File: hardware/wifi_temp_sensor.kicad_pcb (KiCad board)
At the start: 2 copper layers, 50.8 x 45.7 mm, 12 parts, among them J1 USB_B_Mini, J2 ESP8266, J3 TempSensor, J4 Prog, J5 Aux_I2C, SW1 BootMode, U2 AZ1117-3.3

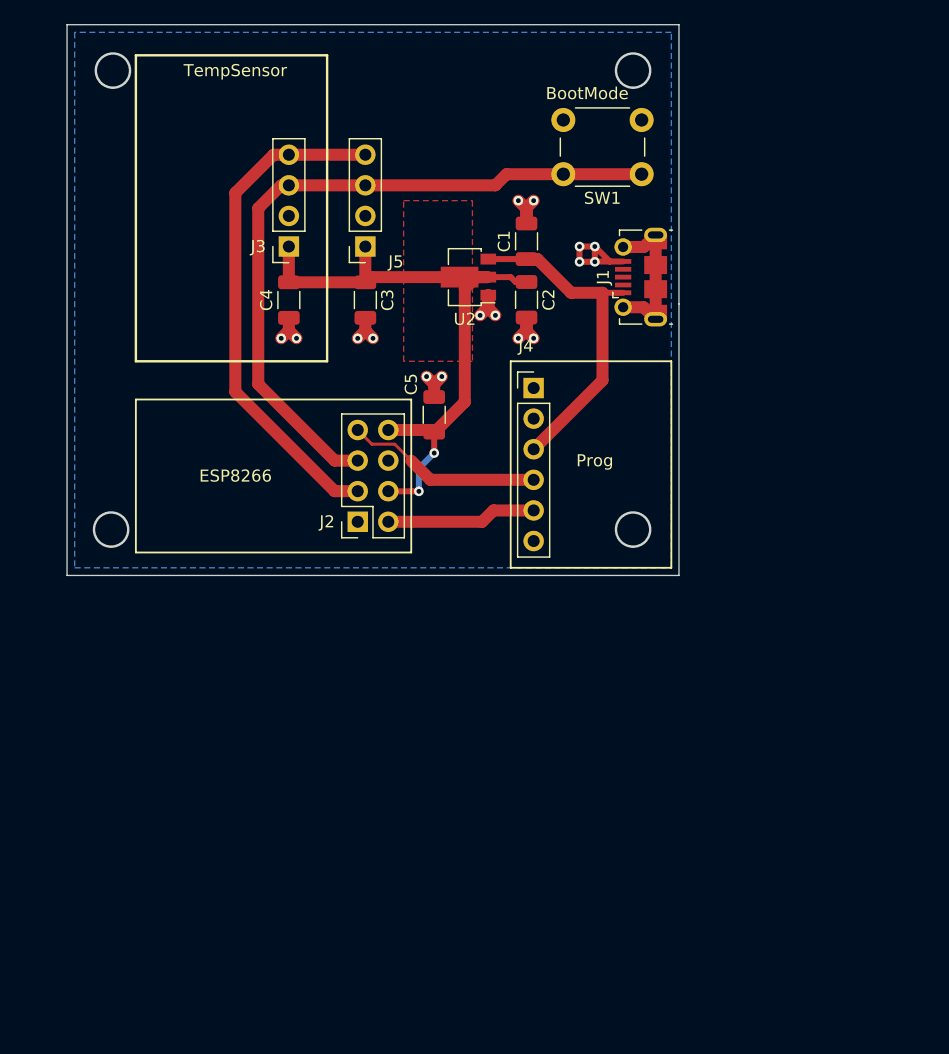
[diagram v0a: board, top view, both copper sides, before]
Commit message: manual merge from esp32_msf_rcnotes
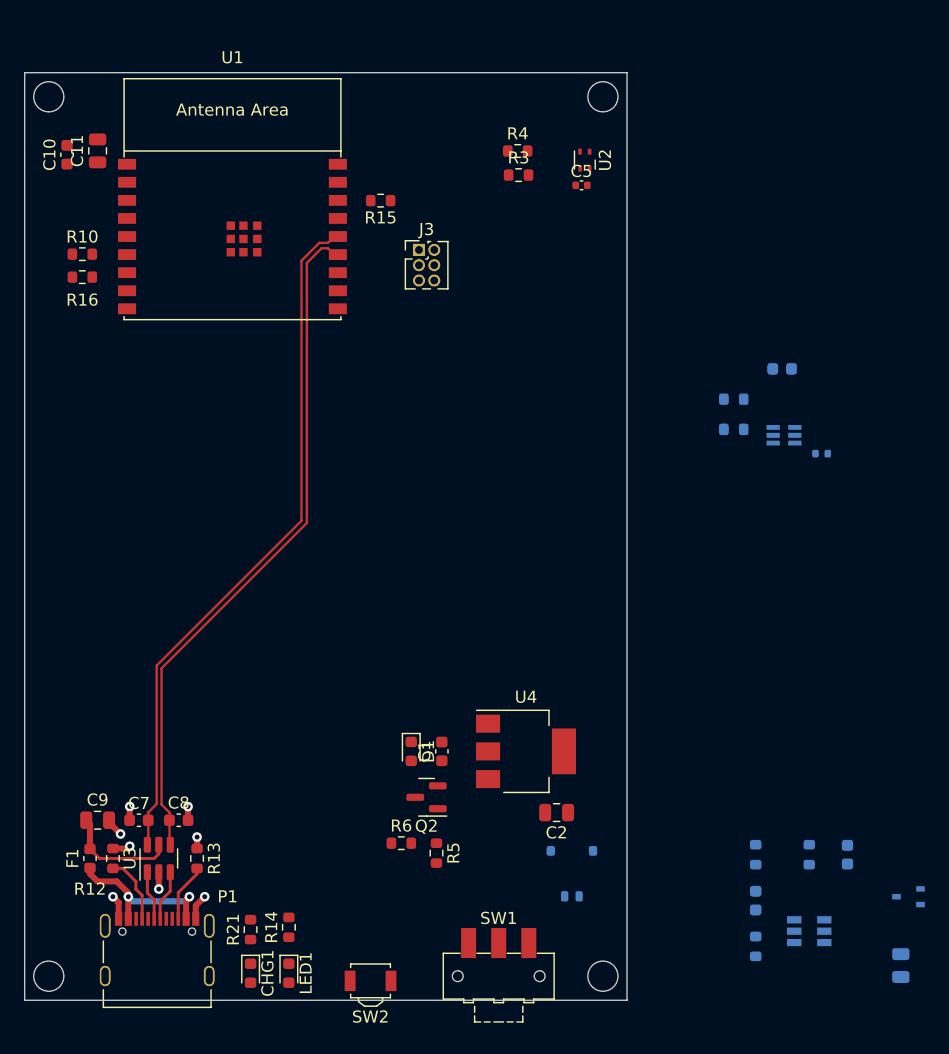
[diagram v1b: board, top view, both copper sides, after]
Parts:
- removed J1: USB_B_Mini, Connector_USB:USB_Micro-B_Molex-105017-0001
- removed J4: Prog, Connector_PinHeader_2.54mm:PinHeader_1x06_P2.54mm_Vertical
- removed J5: Aux_I2C, Connector_PinSocket_2.54mm:PinSocket_1x04_P2.54mm_Vertical
- added C10: 100nF, Capacitor_SMD:C_0603_1608Metric, F.Cu at (183.5, 35.6)
- added C11: 10uF, Capacitor_SMD:C_0805_2012Metric, F.Cu at (186.1, 35.2)
- added C12: 100nF, Capacitor_SMD:C_0603_1608Metric, B.Cu at (248.3, 93.7)
- added C6: 10uF, Capacitor_SMD:C_0805_2012Metric, B.Cu at (252.7, 102.9)
- added C7: 22pF, Capacitor_SMD:C_0603_1608Metric, F.Cu at (189.5, 90.8)
- added C8: 22pF, Capacitor_SMD:C_0603_1608Metric, F.Cu at (192.8, 90.8)
- added C9: 10uF, Capacitor_SMD:C_0805_2012Metric, F.Cu at (186.1, 90.8)
- added CHG1: LED_Small, LED_SMD:LED_0603_1608Metric, F.Cu at (198.8, 103.5)
- added D1: D_Schottky, Diode_SMD:D_0603_1608Metric, F.Cu at (212.1, 85.1)
- added F1: Polyfuse_Small, Fuse:Fuse_0603_1608Metric, F.Cu at (185.4, 94.0)
- added IC2: BQ21040DBVR, TI BQ21040:SOT95P280X145-6N, B.Cu at (245.1, 100.0)
- added LED1: LED_Small, LED_SMD:LED_0603_1608Metric, F.Cu at (201.9, 103.5)
- added P1: USB_C_Plug_USB2.0, Connector_USB:USB_C_Receptacle_Palconn_UTC16-G, F.Cu at (191.0, 101.5)
- added Q1: SSM6L09FUTE85LF, SamacSys_parts:SOT65P210X120-6N, B.Cu at (243.0, 58.9)
- added Q2: AO3401A, Package_TO_SOT_SMD:SOT-23, F.Cu at (213.4, 88.9)
- added Q3: BSS214NW, Package_TO_SOT_SMD:SOT-323_SC-70, B.Cu at (253.4, 97.2)
- added R1: 100K, Resistor_SMD:R_0603_1608Metric, B.Cu at (238.9, 55.9)
- added R10: 10k, Resistor_SMD:R_0603_1608Metric, F.Cu at (184.8, 43.8)
- added R11: 100K, Resistor_SMD:R_0402_1005Metric, B.Cu at (246.2, 60.4)
- added R12: 5.1K, Resistor_SMD:R_0603_1608Metric, F.Cu at (187.3, 94.0)
- added R13: 5.1K, Resistor_SMD:R_0603_1608Metric, F.Cu at (194.3, 94.0)
- added R14: 33R, Resistor_SMD:R_0603_1608Metric, F.Cu at (201.9, 99.7)
- added R15: 10k, Resistor_SMD:R_0603_1608Metric, F.Cu at (209.6, 39.4)
- added R16: 10k, Resistor_SMD:R_0603_1608Metric, F.Cu at (184.8, 45.7)
- added R19: 33K, Resistor_SMD:R_0603_1608Metric, B.Cu at (240.7, 93.7)
- added R2: 100K, Resistor_SMD:R_0603_1608Metric, B.Cu at (238.9, 58.4)
- added R20: 10K, Resistor_SMD:R_0603_1608Metric, B.Cu at (245.1, 93.7)
- added R21: 33R, Resistor_SMD:R_0603_1608Metric, F.Cu at (198.8, 99.9)
- added R3: 10k, Resistor_SMD:R_0603_1608Metric, F.Cu at (221.0, 37.2)
- added R4: 10k, Resistor_SMD:R_0603_1608Metric, F.Cu at (220.9, 35.2)
- added R5: 10K, Resistor_SMD:R_0603_1608Metric, F.Cu at (214.2, 93.5)
- added R6: 1K, Resistor_SMD:R_0603_1608Metric, F.Cu at (211.3, 92.7)
- added R9: R_Small, Resistor_SMD:R_0603_1608Metric, B.Cu at (240.7, 101.3)
- added SW2: SW_Push, Button_Switch_SMD:SW_SPST_B3U-3000P, F.Cu at (208.7, 104.1)
- added U1: ESP32-C3-WROOM-02, PCM_Espressif:ESP32-C3-WROOM-02, F.Cu at (197.2, 42.2)
- added U3: WE-TVS-82400102, Package_TO_SOT_SMD:SOT-23-6, F.Cu at (191.1, 94.0)
- added U4: LD1117S33TR_SOT223, Package_TO_SOT_SMD:SOT-223-3_TabPin2, F.Cu at (221.6, 85.1)
- C1: value 10uF -> 1uF; footprint Capacitor_SMD:C_1206_3216Metric -> Capacitor_SMD:C_0603_1608Metric
- C2: value 22uF -> 10uF; footprint Capacitor_SMD:C_1206_3216Metric -> Capacitor_SMD:C_0805_2012Metric
- C3: value C_Small -> 1uF; footprint Capacitor_SMD:C_1206_3216Metric -> Capacitor_SMD:C_0603_1608Metric; moved to B.Cu
- C4: value C_Small -> 100nF; footprint Capacitor_SMD:C_1206_3216Metric -> Capacitor_SMD:C_0603_1608Metric; moved to B.Cu
- C5: value C_Small -> 100nF; footprint Capacitor_SMD:C_1206_3216Metric -> Capacitor_SMD:C_0402_1005Metric
- J2: value ESP8266 -> Batt_Conn; footprint Connector_PinSocket_2.54mm:PinSocket_2x04_P2.54mm_Vertical -> Connector_JST:JST_ACH_BM02B-ACHSS-GAN-ETF_1x02-1MP_P1.20mm_Vertical; moved to B.Cu
- J3: value TempSensor -> Conn_02x03_Odd_Even; footprint Connector_PinSocket_2.54mm:PinSocket_1x04_P2.54mm_Vertical -> Connector_PinHeader_1.27mm:PinHeader_2x03_P1.27mm_Vertical
- SW1: value BootMode -> SW_SPST; footprint Button_Switch_THT:SW_PUSH_6mm -> Button_Switch_SMD:SW_SPDT_CK-JS102011SAQN
- U2: value AZ1117-3.3 -> SHT4x; footprint Package_TO_SOT_SMD:SOT-89-3 -> Sensor_Humidity:Sensirion_DFN-4_1.5x1.5mm_P0.8mm_SHT4x_NoCentralPad
- moved SW1 67.6 mm to (219.3, 103.8), turned to 0 degrees
- moved C3 59.5 mm to (240.7, 97.5)
- moved C1 42.9 mm to (214.6, 85.1)
- moved C2 42.6 mm to (224.2, 90.2), turned to 180 degrees
- moved C4 41.3 mm to (242.9, 53.3), turned to 180 degrees
- moved J2 34.2 mm to (225.4, 95.2), turned to 0 degrees
- moved C5 22.6 mm to (226.2, 38.1), turned to 0 degrees
- moved U2 13.9 mm to (226.5, 36.0), turned to -90 degrees
- moved J3 10.8 mm to (212.7, 43.5), turned to 0 degrees
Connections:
- C1 pad 1: +5V -> Net-(D1-K)
- C3 pad 1: +3.3V -> V_USB
- C4 pad 1: GND -> V_BAT_MEAS
- C4 pad 2: +3.3V -> GND
- J2 pad 2: ESP_Tx -> Net-(J2-Pin_2)
- J3 pad 1: +3.3V -> EN
- J3 pad 2: GND -> +3.3V
- J3 pad 3: SCL -> TXD
- J3 pad 4: SDA -> IO9
- SW1 pad 1: SCL -> Net-(J2-Pin_2)
- SW1 pad 2: GND -> V_BAT
- U2 pad 1: GND -> SDA
- U2 pad 2: +3.3V -> SDC
- U2 pad 3: +5V -> +3.3V
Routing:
- net SCL: track 58.5 -> 0.00 mm
- net D+: track 0.00 -> 57.6 mm
- net D-: track 0.00 -> 56.9 mm
- net +3.3V: track 55.6 -> 0.00 mm, vias 2 -> 0
- net SDA: track 42.2 -> 0.00 mm
- net +5V: track 27.7 -> 0.00 mm
- net GND: track 30.0 -> 11.8 mm, vias 16 -> 8
- net ESP_Rx: track 16.9 -> 0.00 mm
- net Net-(F1-Pad1): track 0.00 -> 13.8 mm, vias 0 -> 2
- net unconnected-(J1-Shield-Pad6): track 13.2 -> 0.00 mm
- net ESP_Tx: track 12.5 -> 0.00 mm
- net V_USB: track 0.00 -> 9.96 mm
- net Net-(P1-CC): track 0.00 -> 5.67 mm
- net Net-(P1-VCONN): track 0.00 -> 4.83 mm
- net Net-(P1-D-): track 0.00 -> 4.22 mm
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- removed copper zone on F.Cu, net +3.3V
- removed copper zone on B.Cu, net GND
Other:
- board size 50.8 x 45.7 mm -> 50 x 77 mm
